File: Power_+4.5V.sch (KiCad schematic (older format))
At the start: 19 parts

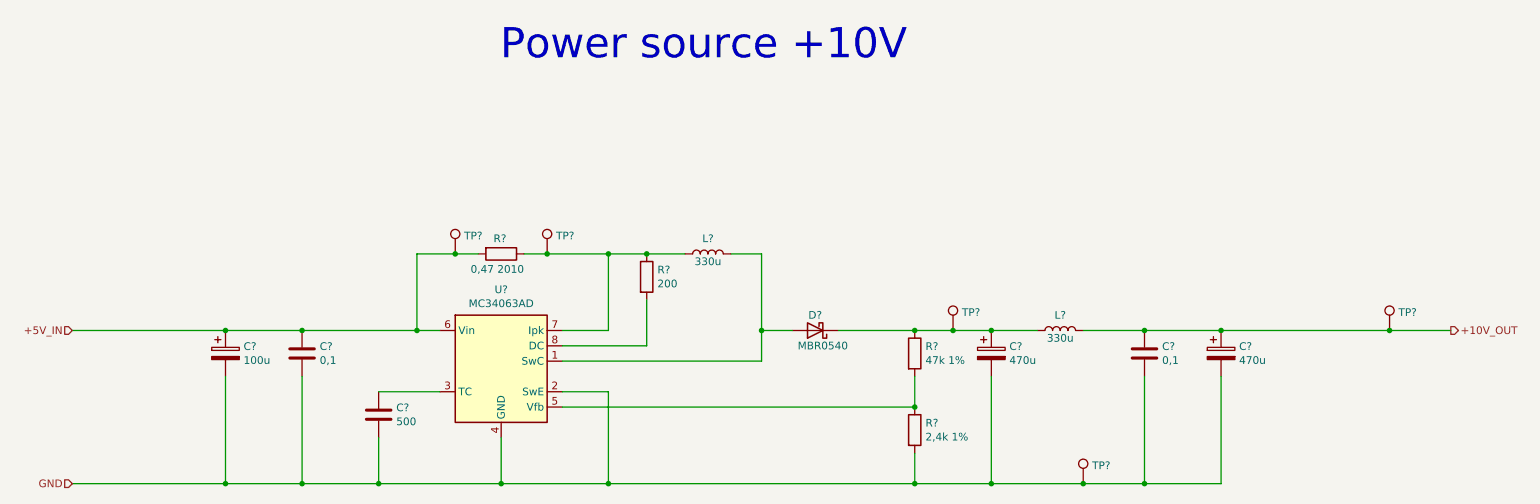
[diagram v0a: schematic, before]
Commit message: Add files via upload
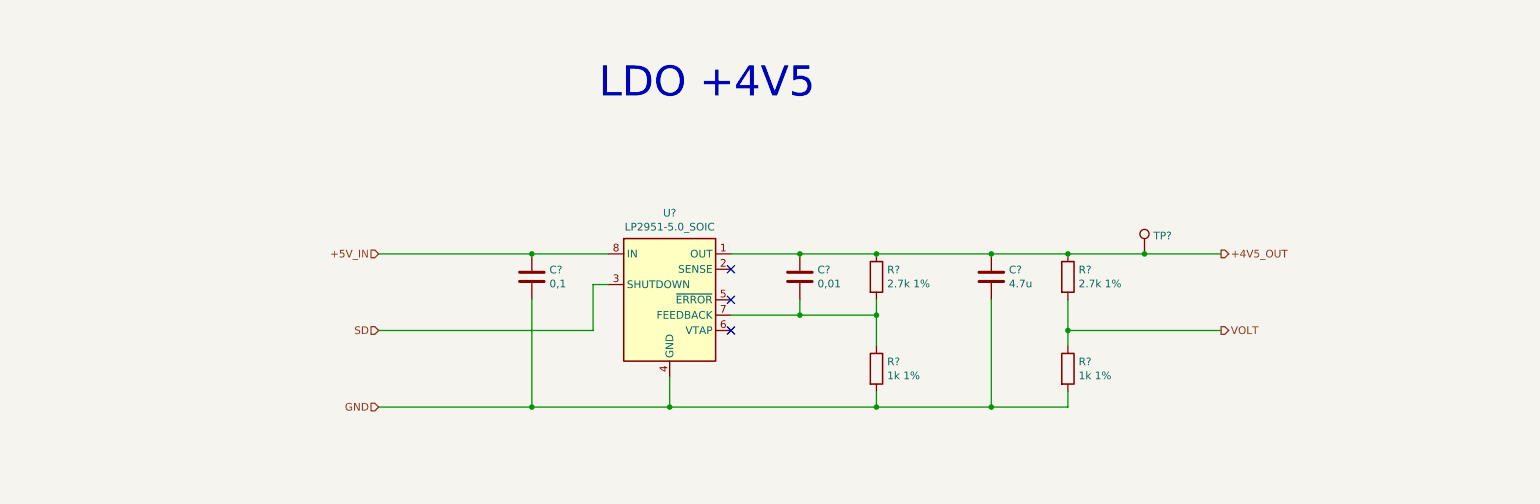
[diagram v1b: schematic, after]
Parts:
- removed C?: 100u, symbol Device:CP
- removed C? (x2): 470u, symbol Device:CP
- removed C? (x2): 0,1, Capacitor_SMD:C_0603_1608Metric_Pad1.08x0.95mm_HandSolder, symbol Device:C
- removed C?: 500, Capacitor_SMD:C_0603_1608Metric_Pad1.08x0.95mm_HandSolder, symbol Device:C
- removed D?: MBR0540, symbol Device:D_Schottky
- removed L? (x2): 330u, symbol Device:L
- removed R?: 47k 1%, Resistor_SMD:R_0603_1608Metric_Pad0.98x0.95mm_HandSolder, symbol Device:R
- removed R?: 0,47 2010, symbol Device:R
- removed R?: 200, Resistor_SMD:R_0603_1608Metric_Pad0.98x0.95mm_HandSolder, symbol Device:R
- removed R?: 2,4k 1%, Resistor_SMD:R_0603_1608Metric_Pad0.98x0.95mm_HandSolder, symbol Device:R
- removed TP? (x4): TestPoint, symbol Connector:TestPoint
- removed U?: MC34063AD, Package_SO:SOIC-8_3.9x4.9mm_P1.27mm, symbol Regulator_Switching:MC34063AD
- added C?: 4.7u, Capacitor_SMD:C_1206_3216Metric_Pad1.33x1.80mm_HandSolder, symbol Device:C
- added C?: 0,1, Capacitor_SMD:C_0603_1608Metric_Pad1.08x0.95mm_HandSolder, symbol Device:C
- added C?: 0,01, Capacitor_SMD:C_0603_1608Metric_Pad1.08x0.95mm_HandSolder, symbol Device:C
- added R? (x2): 1k 1%, Resistor_SMD:R_0603_1608Metric_Pad0.98x0.95mm_HandSolder, symbol Device:R
- added R? (x2): 2.7k 1%, Resistor_SMD:R_0603_1608Metric_Pad0.98x0.95mm_HandSolder, symbol Device:R
- added U?: LP2951-5.0_SOIC, Package_SO:SOIC-8_3.9x4.9mm_P1.27mm, symbol Regulator_Linear:LP2951-5.0_SOIC
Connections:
- net +5V_IN: now also C?.1, U?.8 (IN)
- net GND: now also C?.2, C?.2, R?.2, R?.2, U?.4 (GND)
- net +4V5_OUT: now reaches TP?.1
- net +4V5_OUT: now also C?.1, C?.1, R?.1, R?.1, U?.1 (OUT)
- new net: C?.2, R?.1, R?.2, U?.7 (FEEDBACK)
- new net SD: U?.3 (SHUTDOWN)
- new net VOLT: R?.1, R?.2
- no-connect marks 0 -> 3
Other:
- note added: "LDO +4V5"
- note removed: "Power source +10V"
- moved on the sheet: TP?
